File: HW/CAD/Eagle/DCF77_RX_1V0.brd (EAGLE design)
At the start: 98.4 x 89.5 mm, 43 parts, among them IC271 LMH6645MF, J131 2SK3557, J221 2SK3557, Q211 QT26V-77.000k, X101 PHOENIX_1990067_1X8X2MM50_PTS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, X391 PHOENIX_1990067_1X8X2MM50_PTS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

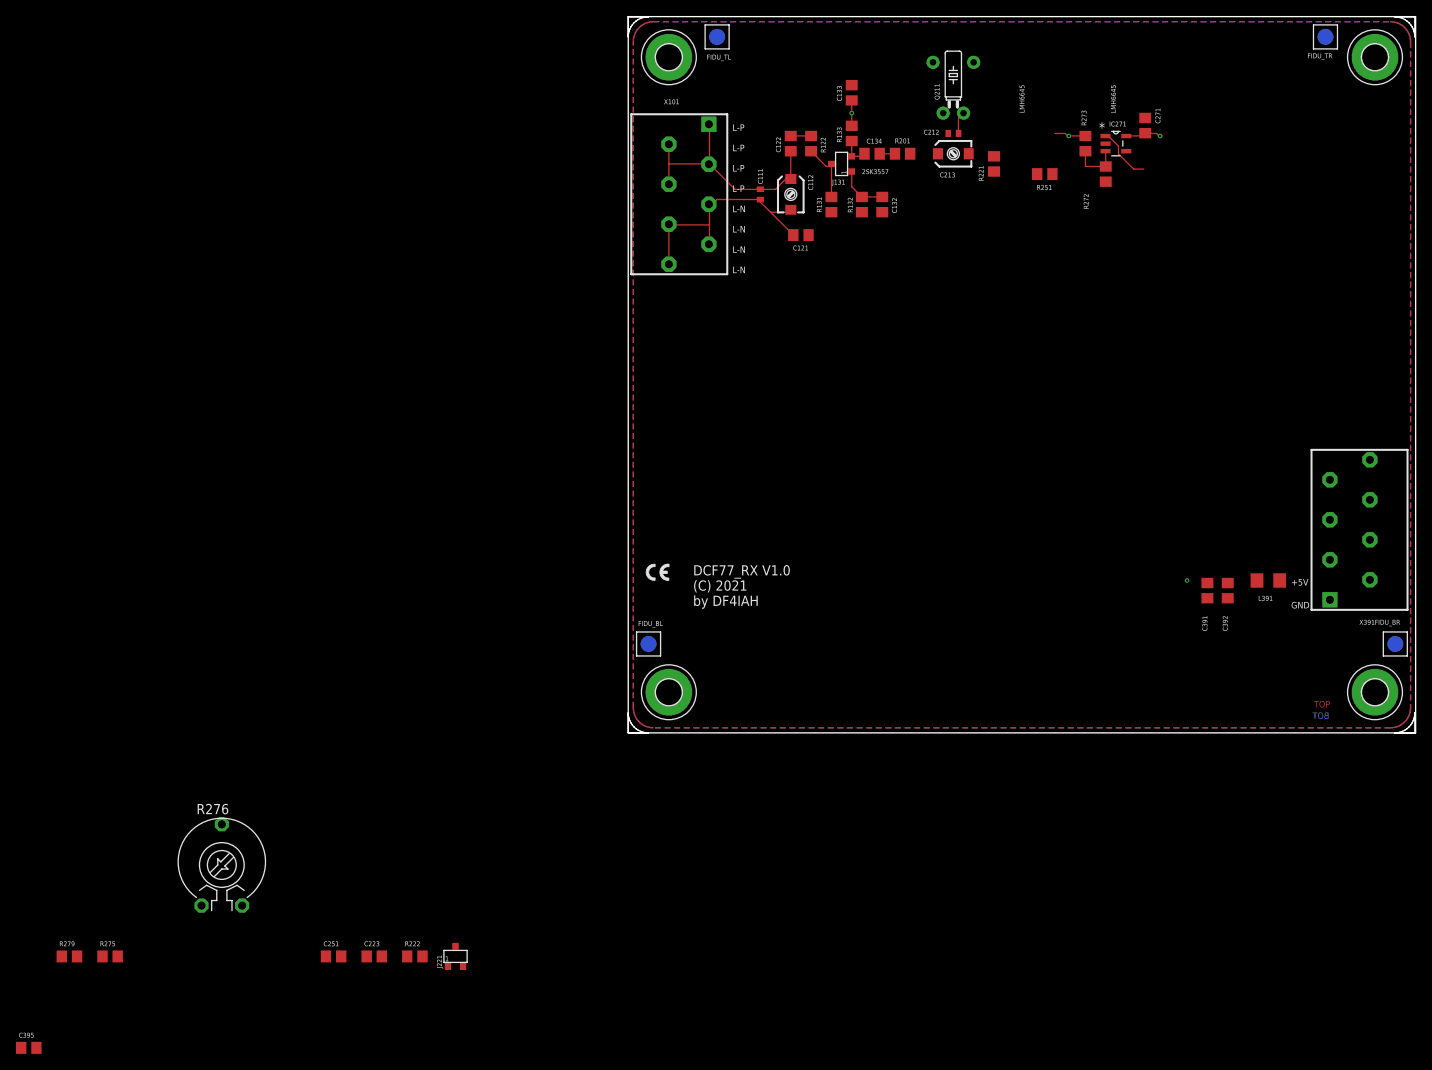
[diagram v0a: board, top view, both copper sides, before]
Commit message: HW - Eagle - Hardware ready for the PCB house V1.0
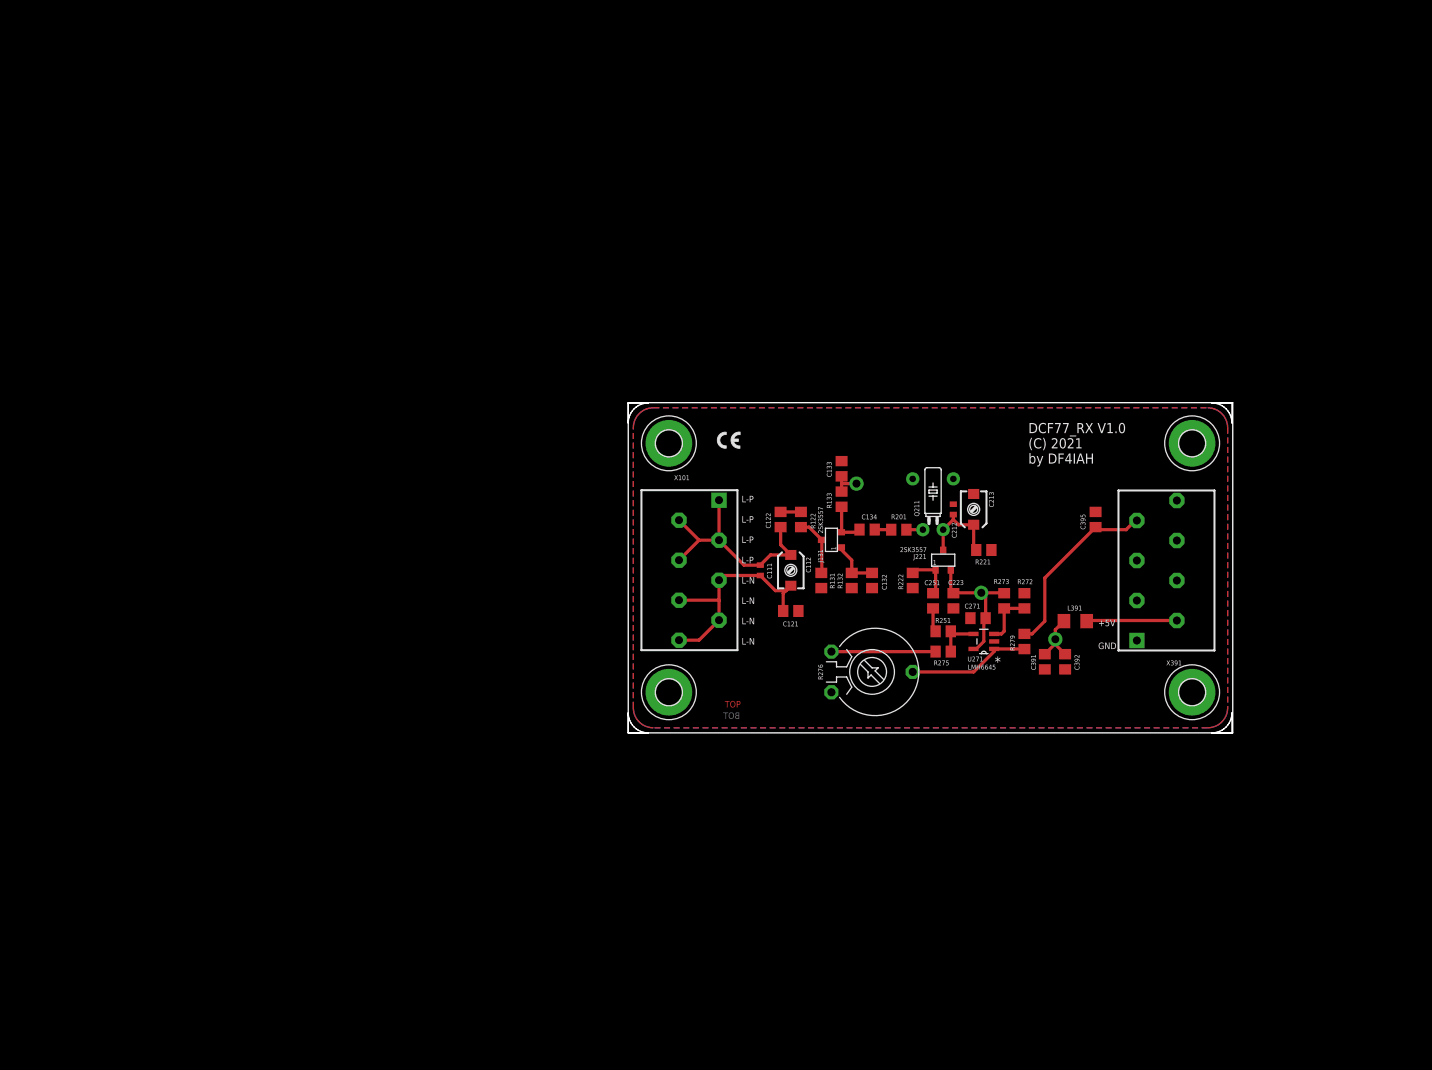
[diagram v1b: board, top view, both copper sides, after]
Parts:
- removed FIDU_BL, FIDU_BR, FIDU_TL, FIDU_TR: (no value), df4iah_fiducial:FIDUCIAL_MARK_1MM
- removed IC271: LMH6645MF, df4iah_opamp:SOT-23-5
- added U271: LMH6645MF, df4iah_opamp:SOT-23-5
- moved C395 148.8 mm to (58.4, 26.7), turned to 90 degrees
- moved R279 125.7 mm to (49.5, 11.4), turned to 90 degrees
- moved R275 110.9 mm to (39.4, 10.2), turned to 180 degrees
- moved C251 87.1 mm to (38.1, 16.5), turned to 270 degrees
- moved C223 84.9 mm to (40.6, 16.5), turned to 270 degrees
- moved R276 84.8 mm to (30.5, 7.62), turned to 270 degrees
- moved J221 78.5 mm to (39.4, 21.6)
- moved R222 78.0 mm to (35.6, 19.1), turned to 90 degrees
- moved C271 65.0 mm to (43.7, 14.3), turned to 180 degrees
- moved R251 58.5 mm to (39.4, 12.7)
- moved R273 58.0 mm to (47.0, 16.5)
- moved R272 54.3 mm to (49.5, 16.5), turned to 270 degrees
- moved H1513 53.4 mm to (70.5, 36.2)
- moved Q211 52.1 mm to (38.1, 25.4)
- moved R221 48.3 mm to (44.5, 22.9), turned to 180 degrees
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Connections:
- net N$2 renamed N211
- net +5V: now also U271.5; no longer IC271.5
- net GND: now also U271.2; no longer IC271.2
- net N271: now also U271.1; no longer IC271.1
- net N272: now also U271.3; no longer IC271.3
- net N273: now also U271.4; no longer IC271.4
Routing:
- net DIG_OUT: track 0.00 -> 23.3 mm
- net +5V: track 11.6 -> 28.8 mm, vias 4 -> 3
- net N275: track 0.00 -> 13.0 mm
- net N391: track 0.00 -> 11.3 mm
- net N221: track 2.80 -> 11.1 mm
- net N271: track 7.06 -> 15.3 mm
- net N222: track 0.00 -> 6.08 mm
- net N273: track 0.00 -> 5.51 mm
- net N251: track 0.00 -> 2.99 mm
- net N133: track 3.70 -> 6.31 mm
- net N211: track 0.00 -> 2.06 mm
- net N101: track 31.3 -> 29.9 mm
- net N102: track 30.6 -> 29.4 mm
- removed copper zone on layer 14, net +3V3
- removed copper zone on layer 15, net GND
- removed copper zone on layer 2, net GND
- removed copper zone on layer 3, net GND
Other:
- board size 98.4 x 89.5 mm -> 75.6 x 41.3 mm
- board text removed: "L14"
- board text removed: "L15"
- board text removed: "L2"
- board text removed: "L3"
